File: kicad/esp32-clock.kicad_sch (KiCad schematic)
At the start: 29 parts, among them J1 Conn_01x07_Socket, Q1 BCW66G, Q2 BCW66G, SW1 RESET, SW2 BOOT, U1 ESP32-PICO-V3, U2 CH340C

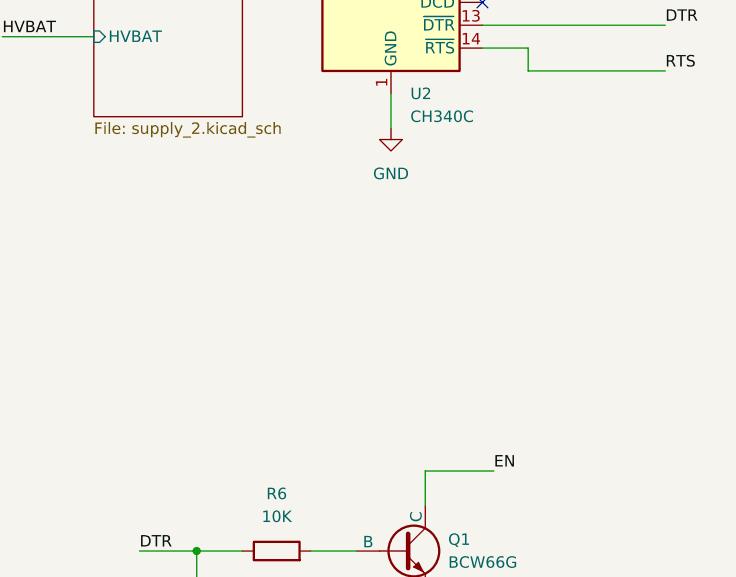
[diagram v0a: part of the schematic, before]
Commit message: init
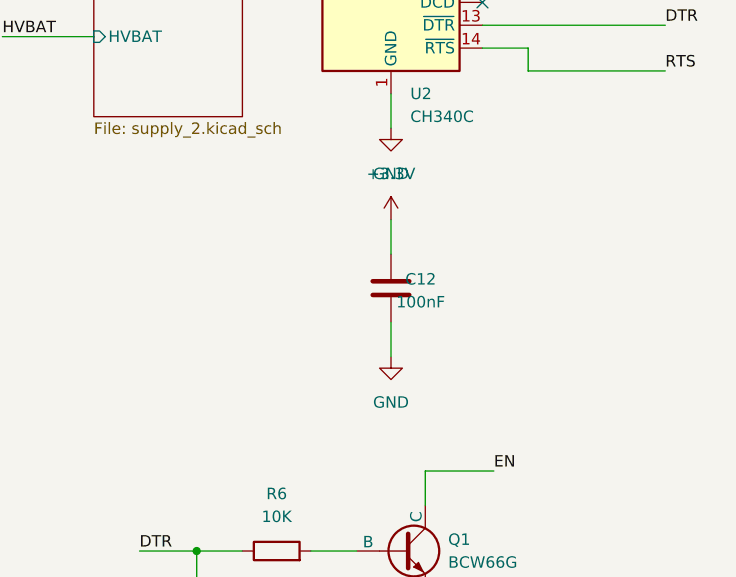
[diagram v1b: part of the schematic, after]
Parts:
- added C12: 100nF, Capacitor_SMD:C_0805_2012Metric, symbol Device:C
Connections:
- net +3.3V: now also C12.1
- net GND: now also C12.2
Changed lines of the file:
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@@
+	)
+	(symbol
+		(lib_id "Device:C")
+		(at 237.49 88.9 0)
+		(unit 1)
+		(exclude_from_sim no)
+		(in_bom yes)
+		(on_board yes)
+		(dnp no)
+		(fields_autoplaced yes)
+		(property "Reference" "C12"
+			(at 240.792 87.9152 0)
+			(effects
+				(font
+					(size 1.27 1.27)
+				)
+			)
+		)
+		(property "Value" "100nF"
+			(at 240.792 90.4552 0)
+			(effects
+				(font
+					(size 1.27 1.27)
+				)
+			)
+		)
+		(property "Footprint" "Capacitor_SMD:C_0805_2012Metric"
+			(at 235.9152 88.9 0)
+			(effects
+				(font
+					(size 1.27 1.27)
+				)
+				(hide yes)
+			)
+		)
+		(property "Datasheet" "~"
+			(at 237.49 88.9 0)
+			(effects
+				(font
+					(size 1.27 1.27)
+				)
+				(hide yes)
+			)
+		)
+		(property "Description" "Unpolarized capacitor"
+			(at 237.49 88.9 0)
+			(effects
+				(font
+					(size 1.27 1.27)
+				)
+				(hide yes)
+			)
+		)
+		(pin "1"
+		)
+		(pin "2"
+		)
+		(instances
+			(project "esp32-clock"
+				(path "/705cc6fa-d5d2-496f-be92-82c69a6f5679"
+					(reference "C12")
+					(unit 1)
+				)
+			)
+		)
+	)
+	(symbol
+		(lib_id "power:+3.3V")
+		(at 237.49 81.28 0)
+		(unit 1)
+		(exclude_from_sim no)
+		(in_bom yes)
+		(on_board yes)
+		(dnp no)
+		(fields_autoplaced yes)
+		(property "Reference" "#PWR030"
+			(at 237.49 85.09 0)
+			(effects
+				(font
+					(size 1.27 1.27)
+				)
+				(hide yes)
+			)
+		)
+		(property "Value" "+3.3V"
+			(at 237.49 76.2 0)
+			(effects
+				(font
+					(size 1.27 1.27)
+				)
+			)
+		)
+		(property "Footprint" ""
+			(at 237.49 81.28 0)
+			(effects
+				(font
+					(size 1.27 1.27)
+				)
+				(hide yes)
+			)
+		)
+		(property "Datasheet" ""
+			(at 237.49 81.28 0)
+			(effects
+				(font
+					(size 1.27 1.27)
+				)
+				(hide yes)
+			)
+		)
+		(property "Description" "Power symbol creates a global label with name \"+3.3V\""
+			(at 237.49 81.28 0)
+			(effects
+				(font
+					(size 1.27 1.27)
+				)
+				(hide yes)
+			)
+		)
+		(pin "1"
+		)
+		(instances
+			(project "esp32-clock"
+				(path "/705cc6fa-d5d2-496f-be92-82c69a6f5679"
+					(reference "#PWR030")
+					(unit 1)
+				)
+			)
+		)
+	)
+	(symbol
+		(lib_id "power:GND")
+		(at 237.49 96.52 0)
+		(unit 1)
+		(exclude_from_sim no)
+		(in_bom yes)
+		(on_board yes)
+		(dnp no)
+		(fields_autoplaced yes)
+		(property "Reference" "#PWR031"
+			(at 237.49 102.87 0)
+			(effects
+				(font
+					(size 1.27 1.27)
+				)
+				(hide yes)
+			)
+		)
+		(property "Value" "GND"
+			(at 237.49 101.6 0)
+			(effects
+				(font
+					(size 1.27 1.27)
+				)
+			)
+		)
+		(property "Footprint" ""
+			(at 237.49 96.52 0)
+			(effects
+				(font
+					(size 1.27 1.27)
+				)
+				(hide yes)
+			)
+		)
+		(property "Datasheet" ""
+			(at 237.49 96.52 0)
+			(effects
+				(font
+					(size 1.27 1.27)
+				)
+				(hide yes)
+			)
+		)
+		(property "Description" "Power symbol creates a global label with name \"GND\" , ground"
+			(at 237.49 96.52 0)
+			(effects
+				(font
+					(size 1.27 1.27)
+				)
+				(hide yes)
+			)
+		)
+		(pin "1"
+		)
+		(instances
+			(project "esp32-clock"
+				(path "/705cc6fa-d5d2-496f-be92-82c69a6f5679"
+					(reference "#PWR031")
+					(unit 1)
+				)
+			)
+		)
 	)
 	(symbol
@@
 	)
 	(embedded_fonts no)
+	(wire
+		(pts
+			(xy 237.49 81.28) (xy 237.49 85.09)
+		)
+		(stroke
+			(width 0)
+			(type default)
+		)
+	)
+	(wire
+		(pts
+			(xy 237.49 92.71) (xy 237.49 96.52)
+		)
+		(stroke
+			(width 0)
+			(type default)
+		)
+	)
 )
